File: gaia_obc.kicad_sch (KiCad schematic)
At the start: 57 parts, among them J1 USB_C_Receptacle_USB2.0_16P, J2 Conn_02x10_Odd_Even, J3 Conn_02x10_Odd_Even, Q1 IRLML6244, SW1 SW_Push, SW2 SW_Push, U1 MCP23017_ML, U2 USBLC6-2P6, U3 ESP32-S3-PICO-1-N8R2

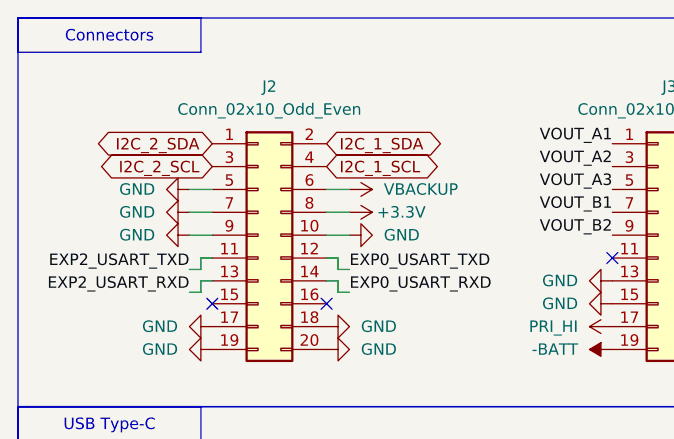
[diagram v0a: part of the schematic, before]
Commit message: obc v1.5
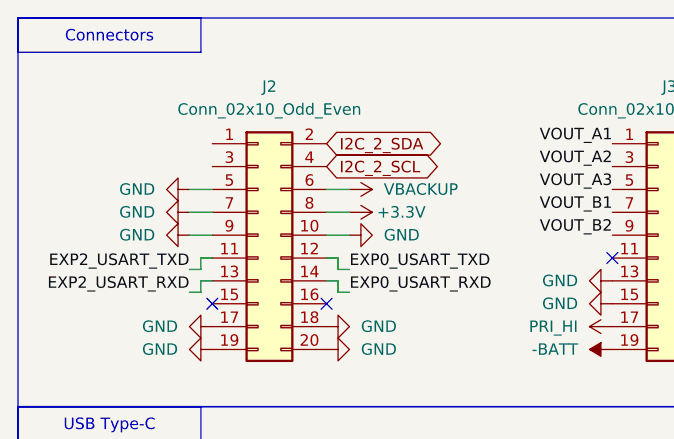
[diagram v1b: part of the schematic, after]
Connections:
- net I2C_1_SCL: no longer J2.4 (Pin_4)
- net I2C_1_SDA: no longer J2.2 (Pin_2)
- net I2C_2_SCL: now also J2.4 (Pin_4); no longer J2.3 (Pin_3)
- net I2C_2_SDA: now also J2.2 (Pin_2); no longer J2.1 (Pin_1)
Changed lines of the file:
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@@
+		)
+	)
+	(global_label "I2C_2_SCL"
+		(shape bidirectional)
+		(at 227.33 60.96 0)
+		(fields_autoplaced yes)
+		(effects
+			(font
+				(size 1.27 1.27)
+			)
+			(justify left)
+		)
+		(property "Intersheetrefs" "${INTERSHEET_REFS}"
+			(at 241.1631 60.96 0)
+			(effects
+				(font
+					(size 1.27 1.27)
+				)
+				(justify left)
+				(hide yes)
+			)
+		)
+	)
+	(global_label "I2C_1_SDA"
+		(shape bidirectional)
+		(at 40.64 140.97 180)
+		(fields_autoplaced yes)
+		(effects
+			(font
+				(size 1.27 1.27)
+			)
+			(justify right)
+		)
+		(property "Intersheetrefs" "${INTERSHEET_REFS}"
+			(at 26.7464 140.97 0)
+			(effects
+				(font
+					(size 1.27 1.27)
+				)
+				(justify right)
+				(hide yes)
+			)
+		)
+	)
+	(global_label "I2C_2_SCL"
+		(shape bidirectional)
+		(at 48.26 30.48 0)
+		(fields_autoplaced yes)
+		(effects
+			(font
+				(size 1.27 1.27)
+			)
+			(justify left)
+		)
+		(property "Intersheetrefs" "${INTERSHEET_REFS}"
+			(at 62.0931 30.48 0)
+			(effects
+				(font
+					(size 1.27 1.27)
+				)
+				(justify left)
+				(hide yes)
+			)
+		)
+	)
+	(global_label "I2C_1_SCL"
+		(shape bidirectional)
+		(at 40.64 143.51 180)
+		(fields_autoplaced yes)
+		(effects
+			(font
+				(size 1.27 1.27)
+			)
+			(justify right)
+		)
+		(property "Intersheetrefs" "${INTERSHEET_REFS}"
+			(at 26.8069 143.51 0)
+			(effects
+				(font
+					(size 1.27 1.27)
+				)
+				(justify right)
+				(hide yes)
+			)
+		)
+	)
+	(global_label "I2C_1_SCL"
+		(shape bidirectional)
+		(at 227.33 55.88 0)
+		(fields_autoplaced yes)
+		(effects
+			(font
+				(size 1.27 1.27)
+			)
+			(justify left)
+		)
+		(property "Intersheetrefs" "${INTERSHEET_REFS}"
+			(at 241.1631 55.88 0)
+			(effects
+				(font
+					(size 1.27 1.27)
+				)
+				(justify left)
+				(hide yes)
+			)
+		)
+	)
+	(global_label "I2C_1_SDA"
+		(shape bidirectional)
+		(at 227.33 53.34 0)
+		(fields_autoplaced yes)
+		(effects
+			(font
+				(size 1.27 1.27)
+			)
+			(justify left)
+		)
+		(property "Intersheetrefs" "${INTERSHEET_REFS}"
+			(at 241.2236 53.34 0)
+			(effects
+				(font
+					(size 1.27 1.27)
+				)
+				(justify left)
+				(hide yes)
+			)
+		)
+	)
+	(global_label "SPI_0_MOSI"
+		(shape bidirectional)
+		(at 227.33 76.2 0)
+		(fields_autoplaced yes)
+		(effects
+			(font
+				(size 1.27 1.27)
+			)
+			(justify left)
+		)
+		(property "Intersheetrefs" "${INTERSHEET_REFS}"
+			(at 242.2517 76.2 0)
+			(effects
+				(font
+					(size 1.27 1.27)
+				)
+				(justify left)
+				(hide yes)
+			)
+		)
+	)
+	(global_label "SPI_0_SCLK"
+		(shape bidirectional)
+		(at 227.33 78.74 0)
+		(fields_autoplaced yes)
+		(effects
+			(font
+				(size 1.27 1.27)
+			)
+			(justify left)
+		)
+		(property "Intersheetrefs" "${INTERSHEET_REFS}"
+			(at 242.4331 78.74 0)
+			(effects
+				(font
+					(size 1.27 1.27)
+				)
+				(justify left)
+				(hide yes)
+			)
+		)
+	)
+	(global_label "SPI_0_MISO"
+		(shape bidirectional)
+		(at 227.33 73.66 0)
+		(fields_autoplaced yes)
+		(effects
+			(font
+				(size 1.27 1.27)
+			)
+			(justify left)
+		)
+		(property "Intersheetrefs" "${INTERSHEET_REFS}"
+			(at 242.2517 73.66 0)
+			(effects
+				(font
+					(size 1.27 1.27)
+				)
+				(justify left)
+				(hide yes)
+			)
 		)
 	)
 	(global_label "I2C_2_SDA"
 		(shape bidirectional)
-		(at 35.56 27.94 180)
-		(fields_autoplaced yes)
-		(effects
-			(font
-				(size 1.27 1.27)
-			)
-			(justify right)
-		)
-		(property "Intersheetrefs" "${INTERSHEET_REFS}"
-			(at 21.6664 27.94 0)
-			(effects
-				(font
-					(size 1.27 1.27)
-				)
-				(justify right)
-				(hide yes)
-			)
-		)
-	)
-	(global_label "I2C_2_SCL"
-		(shape bidirectional)
-		(at 227.33 60.96 0)
-		(fields_autoplaced yes)
-		(effects
-			(font
-				(size 1.27 1.27)
-			)
-			(justify left)
-		)
-		(property "Intersheetrefs" "${INTERSHEET_REFS}"
-			(at 241.1631 60.96 0)
-			(effects
-				(font
-					(size 1.27 1.27)
-				)
-				(justify left)
-				(hide yes)
-			)
-		)
-	)
-	(global_label "I2C_1_SDA"
-		(shape bidirectional)
 		(at 48.26 27.94 0)
 		(fields_autoplaced yes)
@@
 			(effects
 				(font
-					(size 1.27 1.27)
-				)
-				(justify left)
-				(hide yes)
-			)
-		)
-	)
-	(global_label "I2C_1_SDA"
-		(shape bidirectional)
-		(at 40.64 140.97 180)
-		(fields_autoplaced yes)
-		(effects
-			(font
-				(size 1.27 1.27)
-			)
-			(justify right)
-		)
-		(property "Intersheetrefs" "${INTERSHEET_REFS}"
-			(at 26.7464 140.97 0)
-			(effects
-				(font
-					(size 1.27 1.27)
-				)
-				(justify right)
-				(hide yes)
-			)
-		)
-	)
-	(global_label "I2C_2_SCL"
-		(shape bidirectional)
-		(at 35.56 30.48 180)
-		(fields_autoplaced yes)
-		(effects
-			(font
-				(size 1.27 1.27)
-			)
-			(justify right)
-		)
-		(property "Intersheetrefs" "${INTERSHEET_REFS}"
-			(at 21.7269 30.48 0)
-			(effects
-				(font
-					(size 1.27 1.27)
-				)
-				(justify right)
-				(hide yes)
-			)
-		)
-	)
-	(global_label "I2C_1_SCL"
-		(shape bidirectional)
-		(at 40.64 143.51 180)
-		(fields_autoplaced yes)
-		(effects
-			(font
-				(size 1.27 1.27)
-			)
-			(justify right)
-		)
-		(property "Intersheetrefs" "${INTERSHEET_REFS}"
-			(at 26.8069 143.51 0)
-			(effects
-				(font
-					(size 1.27 1.27)
-				)
-				(justify right)
-				(hide yes)
-			)
-		)
-	)
-	(global_label "I2C_1_SCL"
-		(shape bidirectional)
-		(at 227.33 55.88 0)
-		(fields_autoplaced yes)
-		(effects
-			(font
-				(size 1.27 1.27)
-			)
-			(justify left)
-		)
-		(property "Intersheetrefs" "${INTERSHEET_REFS}"
-			(at 241.1631 55.88 0)
-			(effects
-				(font
-					(size 1.27 1.27)
-				)
-				(justify left)
-				(hide yes)
-			)
-		)
-	)
-	(global_label "I2C_1_SDA"
-		(shape bidirectional)
-		(at 227.33 53.34 0)
-		(fields_autoplaced yes)
-		(effects
-			(font
-				(size 1.27 1.27)
-			)
-			(justify left)
-		)
-		(property "Intersheetrefs" "${INTERSHEET_REFS}"
-			(at 241.2236 53.34 0)
-			(effects
-				(font
-					(size 1.27 1.27)
-				)
-				(justify left)
-				(hide yes)
-			)
-		)
-	)
-	(global_label "SPI_0_MOSI"
-		(shape bidirectional)
-		(at 227.33 76.2 0)
-		(fields_autoplaced yes)
-		(effects
-			(font
-				(size 1.27 1.27)
-			)
-			(justify left)
-		)
-		(property "Intersheetrefs" "${INTERSHEET_REFS}"
-			(at 242.2517 76.2 0)
-			(effects
-				(font
-					(size 1.27 1.27)
-				)
-				(justify left)
-				(hide yes)
-			)
-		)
-	)
-	(global_label "SPI_0_SCLK"
-		(shape bidirectional)
-		(at 227.33 78.74 0)
-		(fields_autoplaced yes)
-		(effects
-			(font
-				(size 1.27 1.27)
-			)
-			(justify left)
-		)
-		(property "Intersheetrefs" "${INTERSHEET_REFS}"
-			(at 242.4331 78.74 0)
-			(effects
-				(font
-					(size 1.27 1.27)
-				)
-				(justify left)
-				(hide yes)
-			)
-		)
-	)
-	(global_label "I2C_1_SCL"
-		(shape bidirectional)
-		(at 48.26 30.48 0)
-		(fields_autoplaced yes)
-		(effects
-			(font
-				(size 1.27 1.27)
-			)
-			(justify left)
-		)
-		(property "Intersheetrefs" "${INTERSHEET_REFS}"
-			(at 62.0931 30.48 0)
-			(effects
-				(font
-					(size 1.27 1.27)
-				)
-				(justify left)
-				(hide yes)
-			)
-		)
-	)
-	(global_label "SPI_0_MISO"
-		(shape bidirectional)
-		(at 227.33 73.66 0)
-		(fields_autoplaced yes)
-		(effects
-			(font
-				(size 1.27 1.27)
-			)
-			(justify left)
-		)
-		(property "Intersheetrefs" "${INTERSHEET_REFS}"
-			(at 242.2517 73.66 0)
-			(effects
-				(font
